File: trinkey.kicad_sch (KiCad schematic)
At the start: 27 parts, among them J1 USB_A, SW1 SW_Push_45deg, U1 RP2040, U2 AMS1117-3.3, U3 W25Q128JVS, X1 ABM8-272-T3

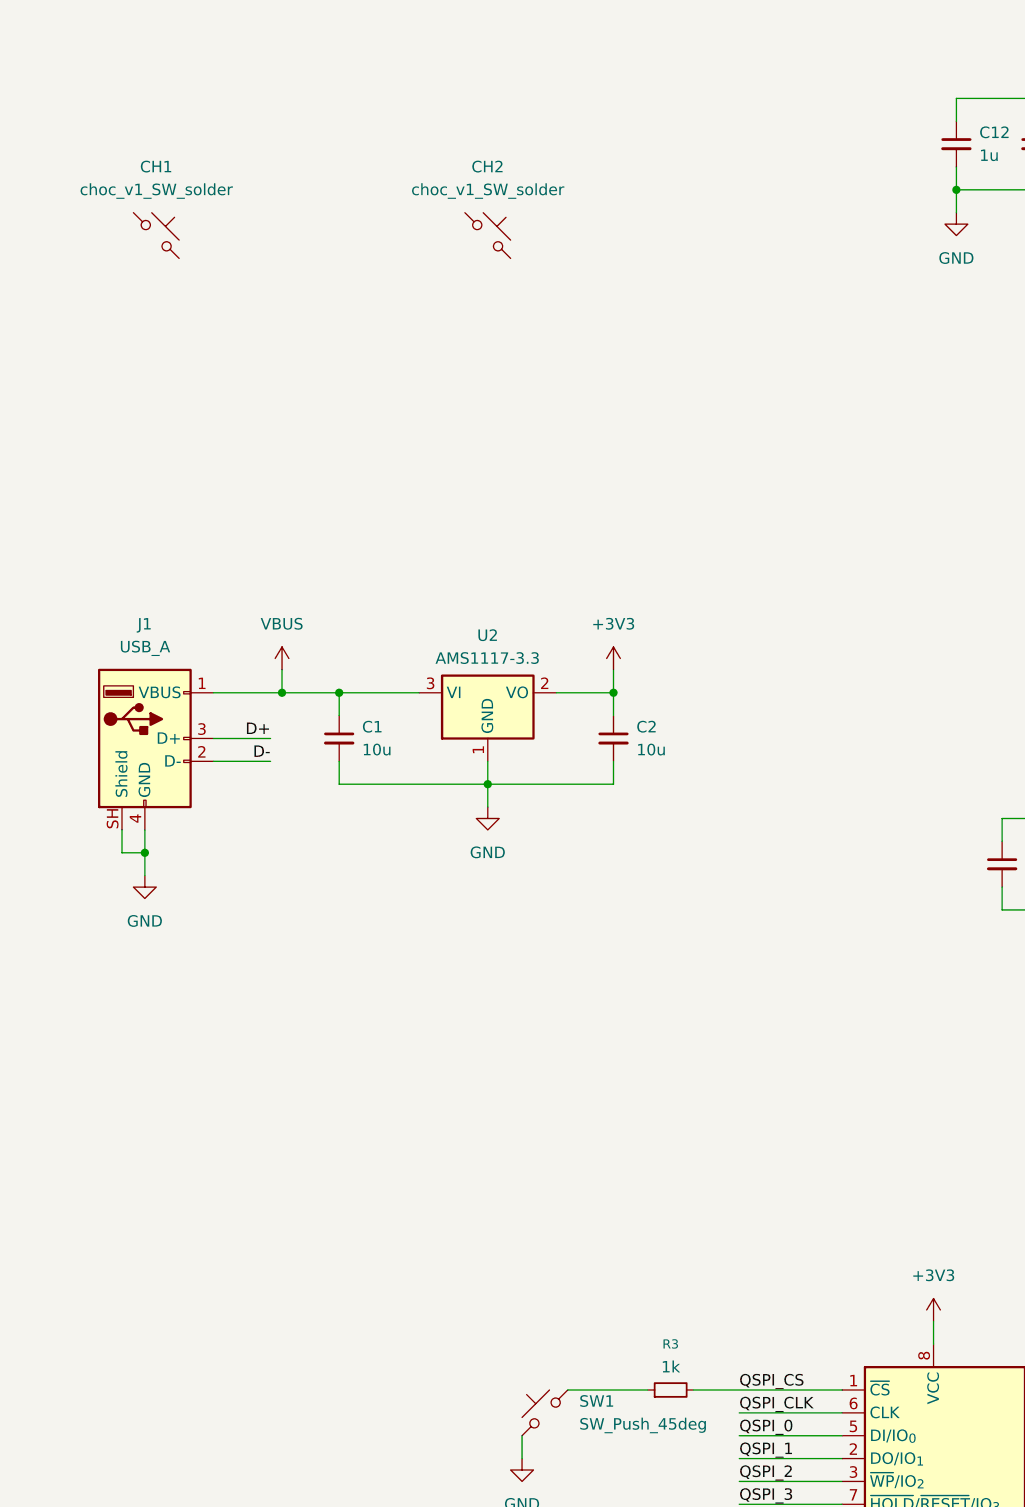
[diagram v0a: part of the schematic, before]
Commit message: feat: packaging ahhhhh
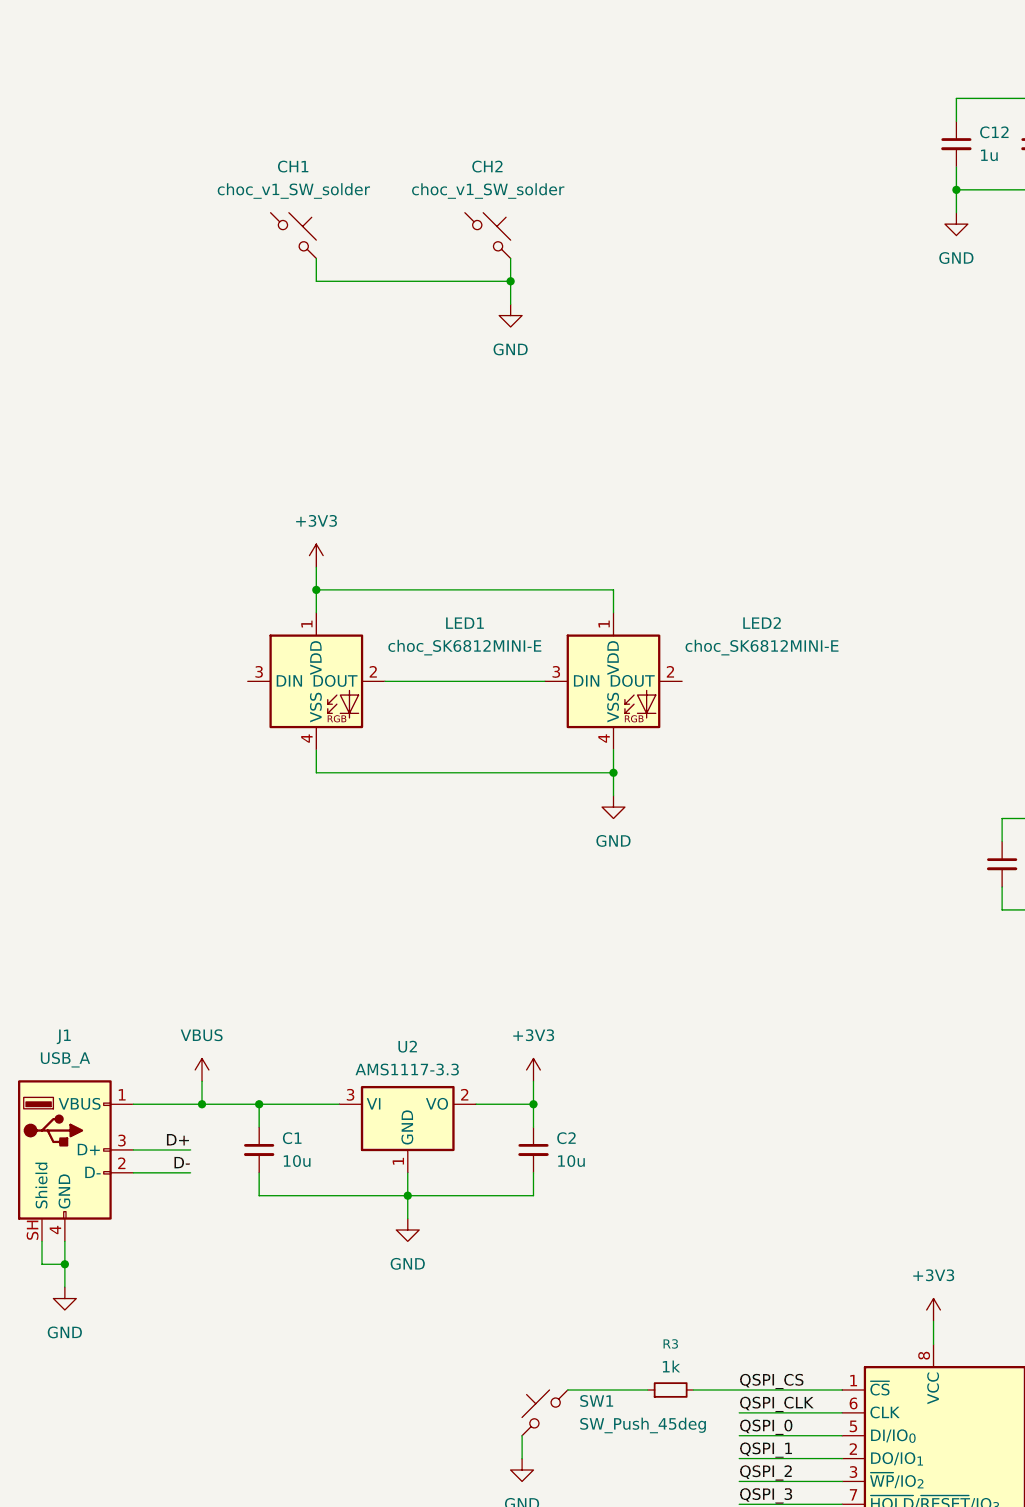
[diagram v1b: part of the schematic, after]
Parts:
- added LED1, LED2: choc_SK6812MINI-E, PCM_marbastlib-choc:LED_choc_6028R, symbol PCM_marbastlib-choc:choc_SK6812MINI-E
- C1, C10, C11, C12, C13, C14, C15, C2, C3, C4, C5, C6, C7, C8, C9: footprint (none) -> Capacitor_SMD:C_0402_1005Metric
- R1, R2, R3, R4: footprint (none) -> Resistor_SMD:R_0402_1005Metric
- SW1: footprint (none) -> TS-1088-AR02016:SW_TS-1088_XNP-L
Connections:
- net +3V3: now also LED1.1 (VDD), LED2.1 (VDD)
- net GND: now also CH1.2, CH2.2, LED1.4 (VSS), LED2.4 (VSS)
- new net: LED1.2 (DOUT), LED2.3 (DIN)
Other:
- moved on the sheet: C1, C2, CH1, J1, U2
